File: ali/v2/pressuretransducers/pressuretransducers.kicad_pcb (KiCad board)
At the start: 4 copper layers, 85 x 76 mm, 191 parts, among them J1 Conn_02x01, J10 Conn_01x02, J11 Conn_01x02, J12 Conn_01x02, J13 Conn_01x02, J14 Conn_01x02, J15 Conn_01x02, J16 Conn_01x02, J17 Conn_01x02, J18 Conn_01x02, J19 Conn_01x02, J2 Conn_01x05, J20 Conn_01x02, J21 Conn_01x02, J22 Conn_01x02, J23 Conn_01x02, J24 Conn_01x02, J25 Conn_01x02, J3 USB_C_Receptacle_USB2.0_16P, J4 Conn_02x09_Counter_Clockwise, J5 Conn_01x15, J6 Screw_Terminal_01x02, J7 Screw_Terminal_01x02, J8 Vertical Ethernet, J9 Conn_01x03, SW1 SKRPANE010, U1 STM32H563RIV6, U2 AP2112K-3.3, U3 LAN8742AI, U4 TJA1462ATK, U5 ADS131M08IRSN, U6 ADS131M08IRSN, Y1 25 MHz, Y2 25 MHz, Y3 8.192 MHz, Y4 8.192 MHz

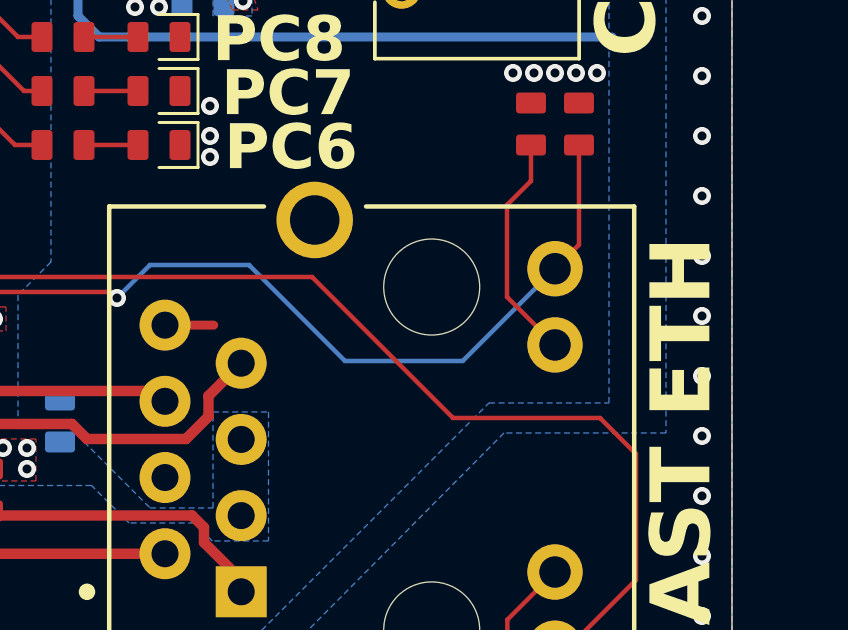
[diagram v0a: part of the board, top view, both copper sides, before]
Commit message: Minor clearance problems
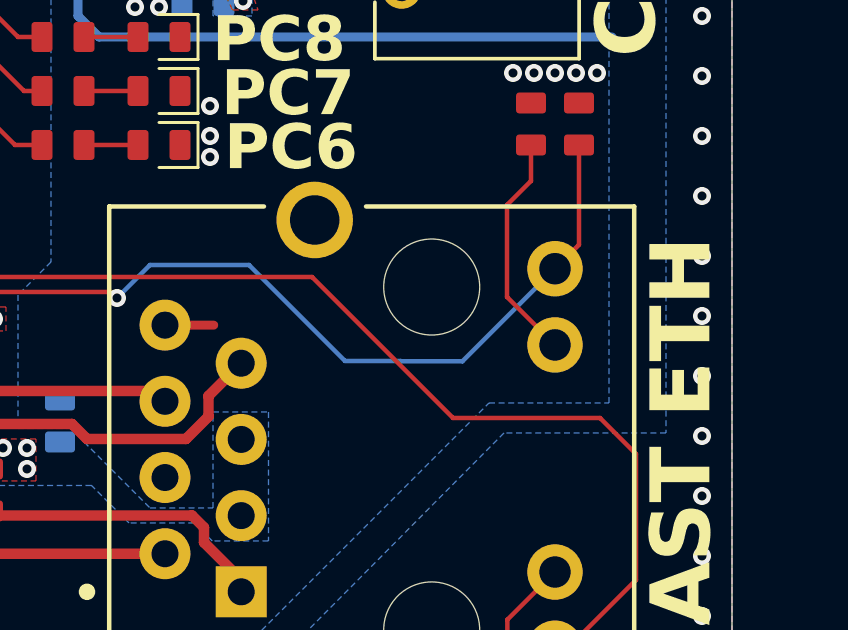
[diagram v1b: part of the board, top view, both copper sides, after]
